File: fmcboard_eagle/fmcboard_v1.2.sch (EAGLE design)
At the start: 108 parts, among them IC1 OPA699ID, IC10 LTC6229IMS8E#TRPBF, IC2 LM2662M_NOPB, IC3 LTC6229IMS8E#TRPBF, IC4 LTC6229IMS8E#TRPBF, IC5 LM358, IC6 OPA699ID, IC7 OPA699ID, IC8 LTC6229IMS8E#TRPBF, IC9 LTC6229IMS8E#TRPBF, J1 8pin, J12 4p-2.54, J2 ASP-134604-01, J3 4p-2.54, J4 4p-2.54, J5 8pin, J6 4p-2.54, J7 4p-2.54, U1 TXS0108EPWR

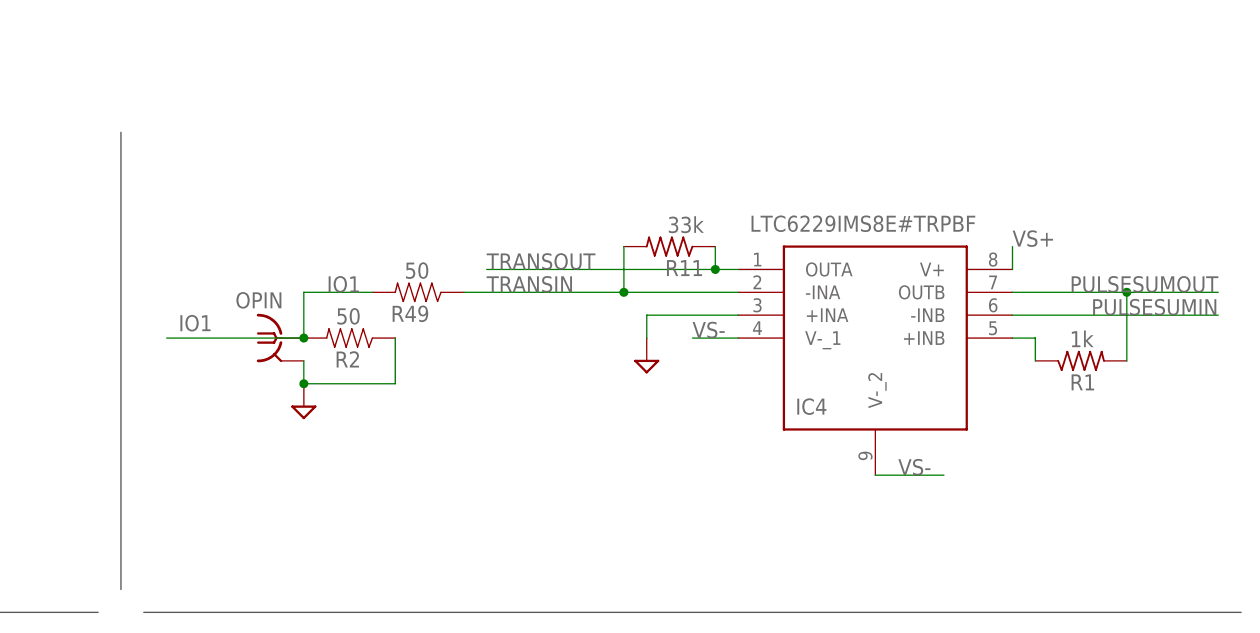
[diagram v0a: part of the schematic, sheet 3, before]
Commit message: Fixes for v1.21, amps etc
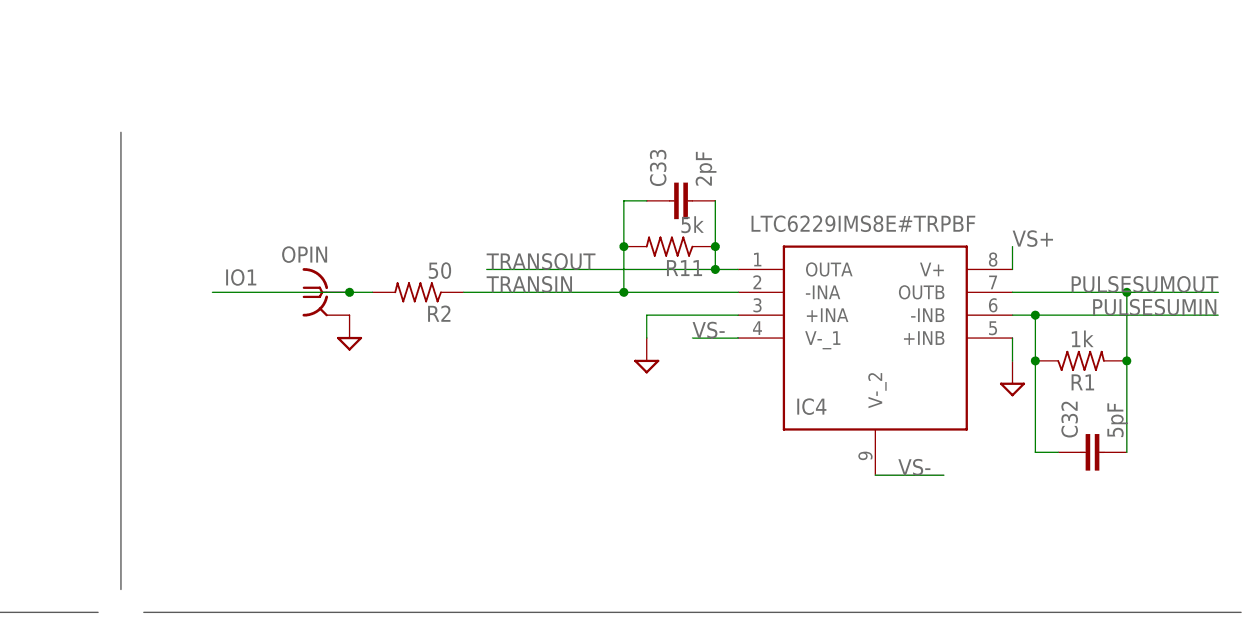
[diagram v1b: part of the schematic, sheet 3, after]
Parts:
- removed R49: 50, SparkFun-Resistors:RESISTORAXIAL-0.3
- added C32, C34, C35, C36, C37: 5pF, SparkFun-Passives:CAP0805
- added C33: 2pF, SparkFun-Passives:CAP0805
- R11: value 33k -> 5k
- R2: device SparkFun-Resistors:RESISTORAXIAL-0.3 -> rcl:R-US_R0805
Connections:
- removed net N$27: IC4.+INB, R1.1
- net GND: now also IC4.+INB; no longer R2.1
- net IO1: no longer R49.2
- net N$12: now also C35.2
- net N$13: now also C34.2
- net N$14: now also C37.1
- net N$4: now also C36.1
- net PULSEINN1: now also C34.1
- net PULSEINN2: now also C36.2
- net PULSEINN3: now also C35.1
- net PULSEINN4: now also C37.2
- net PULSESUMIN: now also C32.1, R1.1
- net PULSESUMOUT: now also C32.2
- net TRANSIN: now also C33.1, R2.1; no longer R49.1
- net TRANSOUT: now also C33.2
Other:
- note removed: "Input goes to a virtual GND at the op amp, so need 50 Ohm? Use _one_ of the 50 Ohm resistors here (?)"
- moved on the sheet: OPIN, R2
